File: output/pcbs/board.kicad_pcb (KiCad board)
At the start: 2 copper layers, 166 x 122.7 mm, 66 parts, among them J1 Jumper, J2 Jumper

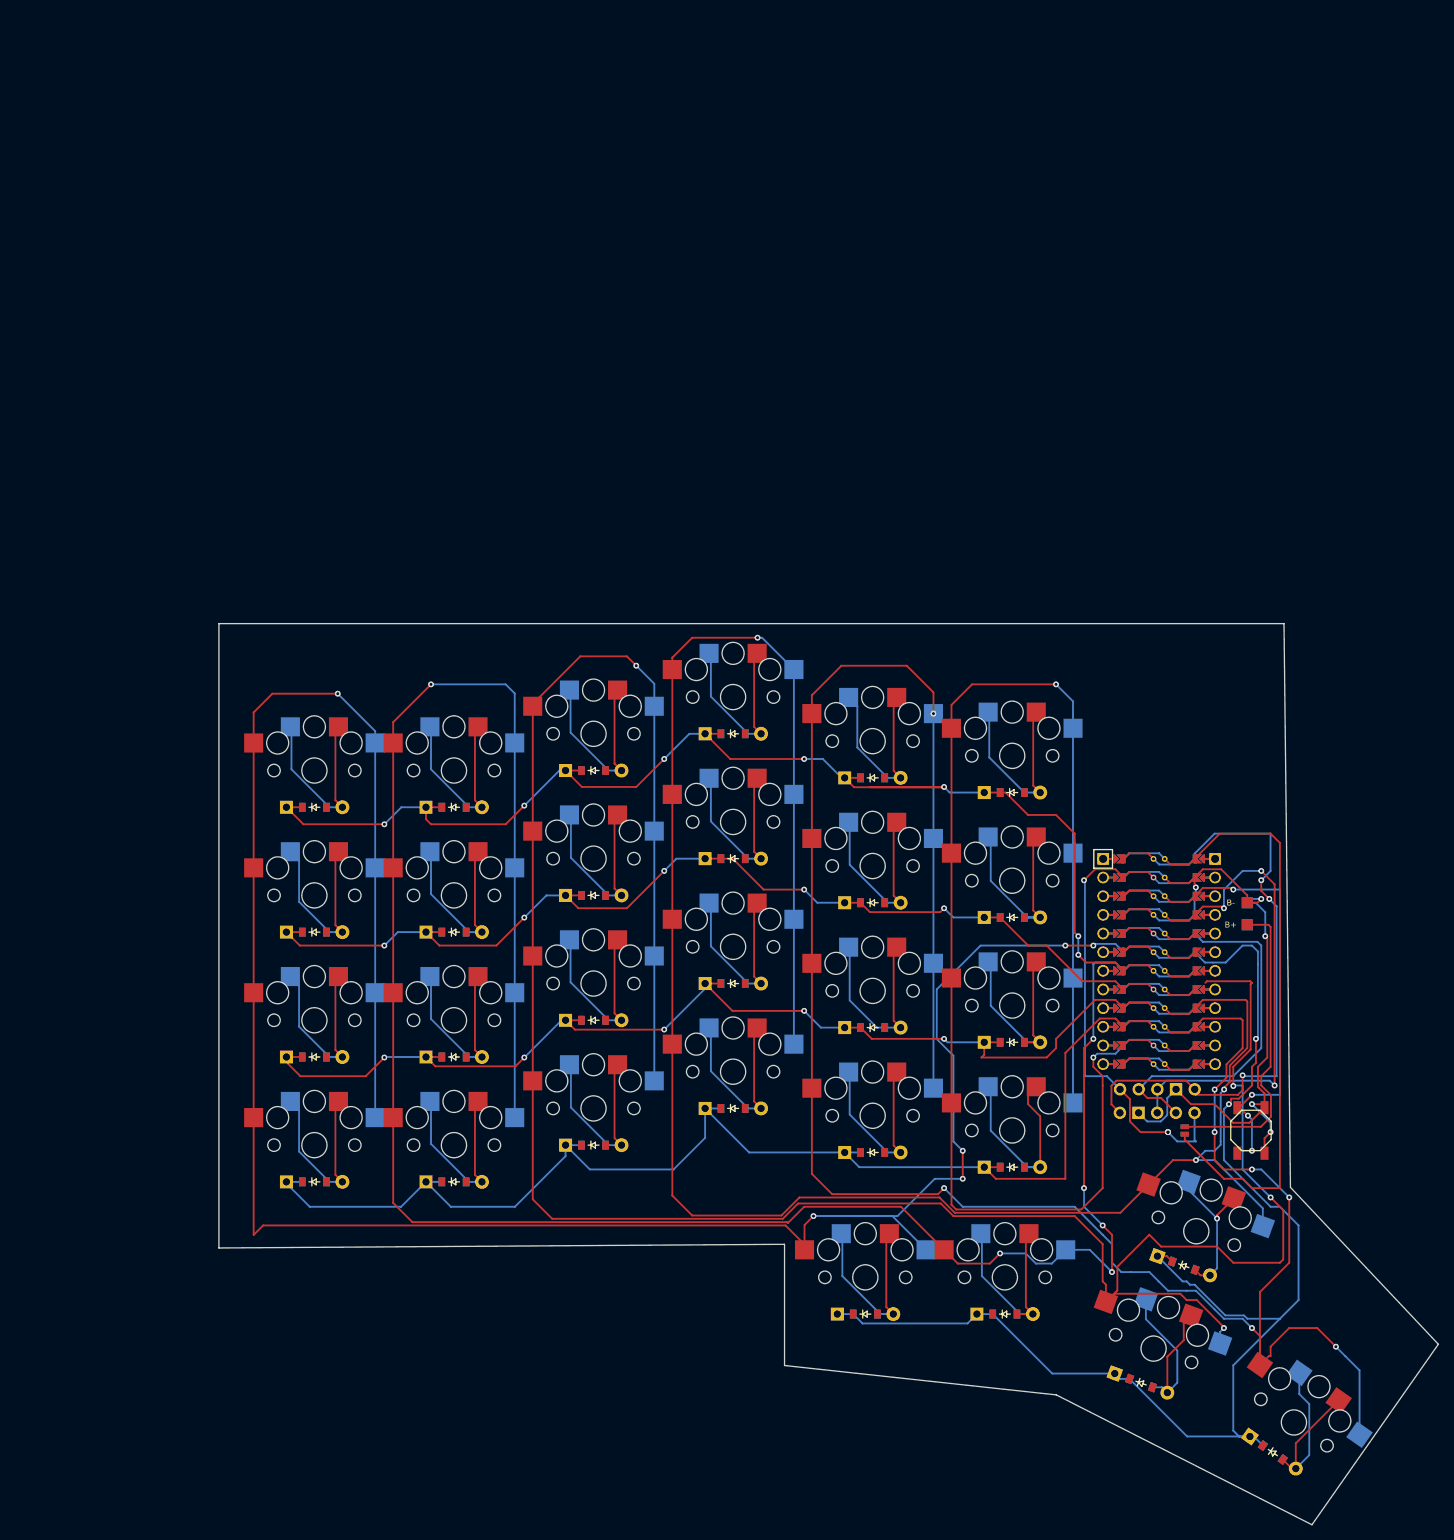
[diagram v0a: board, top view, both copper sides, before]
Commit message: new onoff and placements
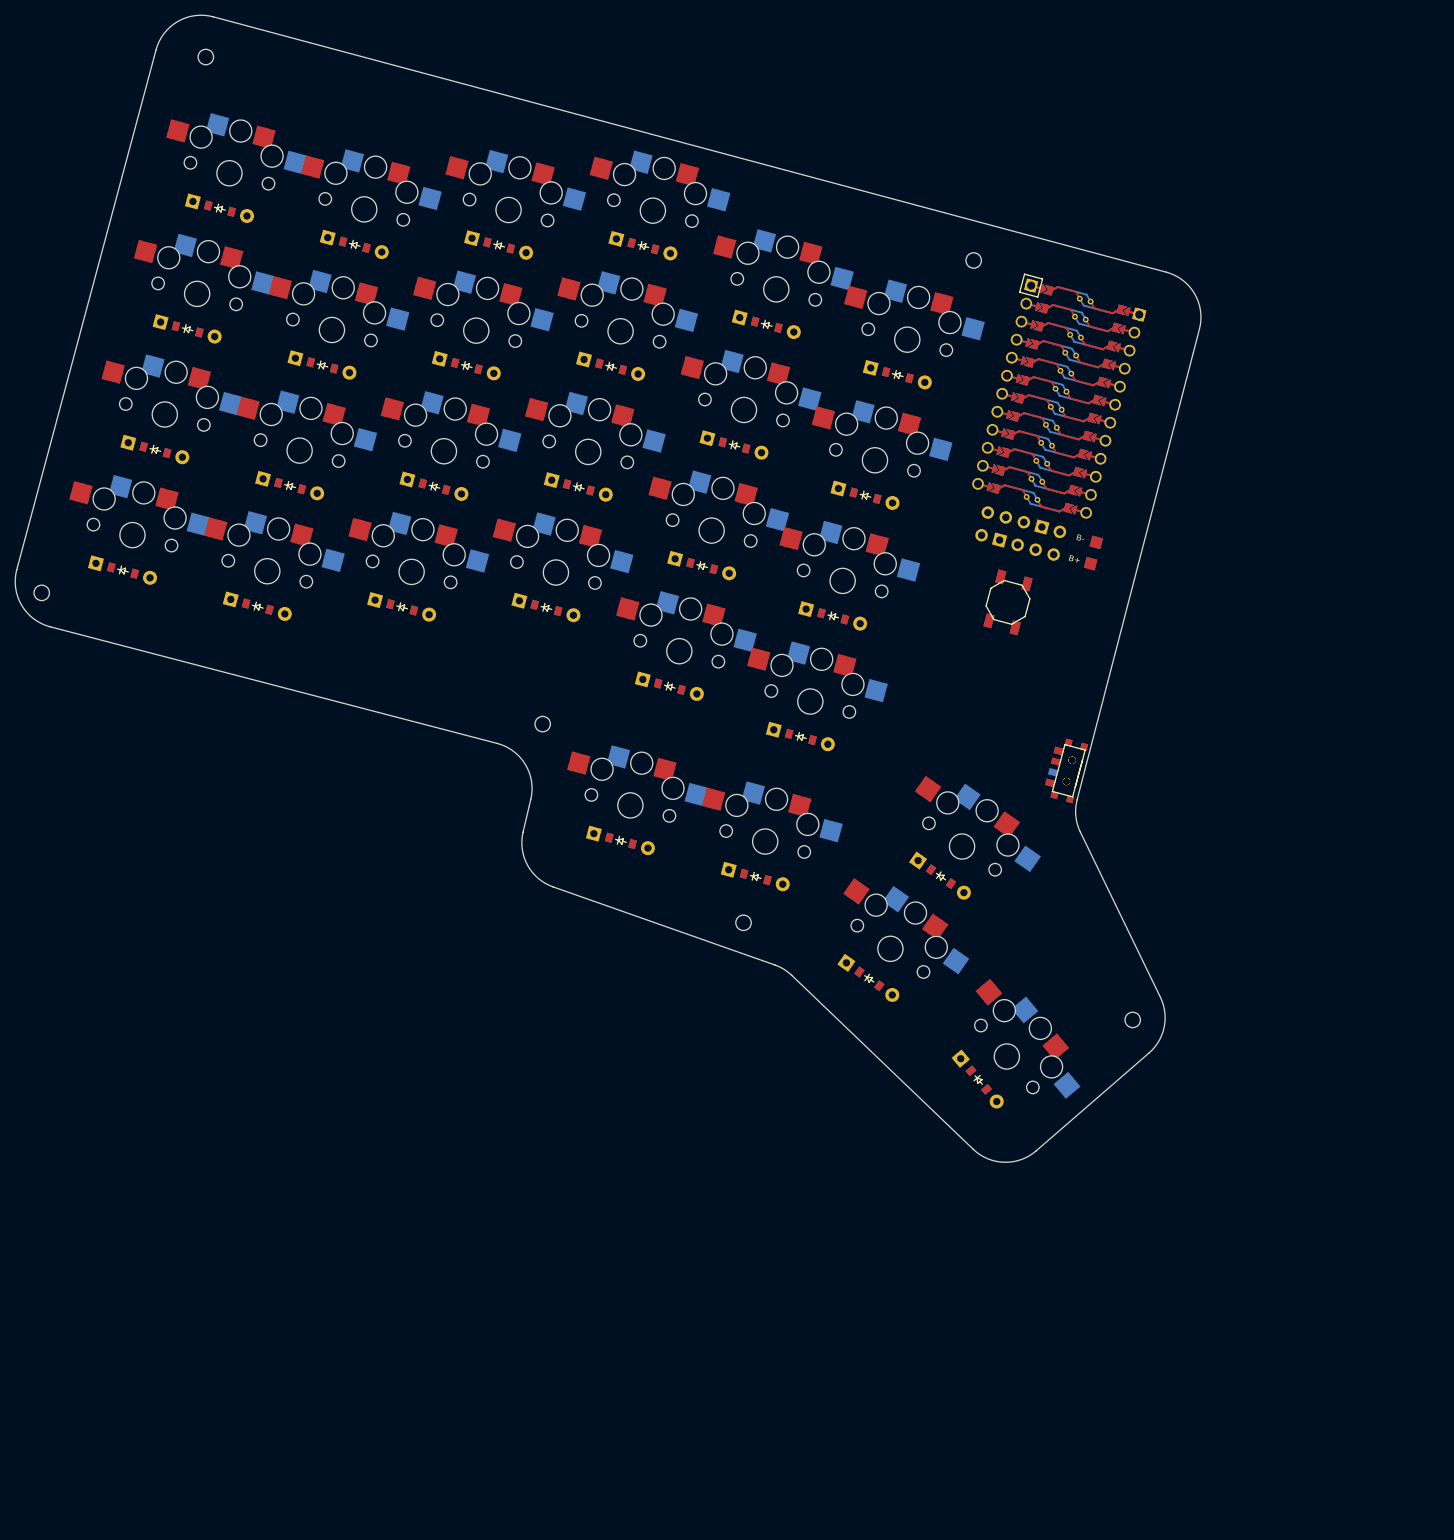
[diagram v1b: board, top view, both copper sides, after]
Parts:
- removed J1, J2: Jumper, lib:Jumper
- added B2: , E73:SW_TACT_ALPS_SKQGABE010, F.Cu at (119.2, 9.16)
- added T1, T2: , E73:SPDT_C128955, F.Cu at (127.5, 32.1)
- moved D1 87.2 mm to (-1.29, 4.83), turned to -15 degrees
- moved S1 86.7 mm to (0.00, 0.00), turned to -15 degrees
- moved D2 85.4 mm to (3.11, -11.6), turned to -15 degrees
- moved S2 84.9 mm to (4.40, -16.4), turned to -15 degrees
- moved D3 83.9 mm to (7.51, -28.0), turned to -15 degrees
- moved S3 83.4 mm to (8.80, -32.8), turned to -15 degrees
- moved D5 82.7 mm to (17.1, 9.75), turned to -15 degrees
- moved D4 82.5 mm to (11.9, -44.4), turned to -15 degrees
- moved S5 82.2 mm to (18.4, 4.92), turned to -15 degrees
- moved S4 82.1 mm to (13.2, -49.3), turned to -15 degrees
- moved OLED1 81.2 mm to (113.9, -2.09), turned to 75 degrees
- moved D6 80.9 mm to (21.5, -6.67), turned to -15 degrees
- moved S6 80.3 mm to (22.8, -11.5), turned to -15 degrees
- moved D7 79.2 mm to (25.9, -23.1), turned to -15 degrees
- moved B1 79.1 mm to (119.2, 9.16), turned to 255 degrees
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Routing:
- net P18: track 333.5 -> 0.00 mm, vias 4 -> 0
- net P20: track 321.2 -> 0.00 mm, vias 6 -> 0
- net P14: track 307.0 -> 0.00 mm, vias 8 -> 0
- net P19: track 297.4 -> 0.00 mm, vias 6 -> 0
- net P15: track 268.2 -> 0.00 mm, vias 3 -> 0
- net P16: track 186.6 -> 0.00 mm, vias 2 -> 0
- net P3: track 178.6 -> 0.00 mm, vias 2 -> 0
- net P4: track 168.4 -> 0.00 mm, vias 7 -> 0
- net P7: track 166.3 -> 0.00 mm
- net P6: track 144.4 -> 0.00 mm, vias 5 -> 0
- net P5: track 136.9 -> 0.00 mm, vias 5 -> 0
- net GND: track 83.7 -> 0.00 mm, vias 5 -> 0
- net P1: track 77.0 -> 0.00 mm, vias 3 -> 0
- net RAW: track 77.0 -> 0.00 mm
- net VCC: track 63.1 -> 0.00 mm, vias 3 -> 0
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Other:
- board size 166 x 122.7 mm -> 161.4 x 156.2 mm
- net class Default added: clearance 0.2, trace_width 0.25, via_dia 0.8, via_drill 0.4
